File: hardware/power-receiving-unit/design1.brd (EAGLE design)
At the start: 55 x 40 mm, 99 parts, among them IC3 TPS54308DDCR, IC4 MCP6486T-E/OT, Q1 BSS138, Q2 SI3481DV, Y1 32MHz, Y2 32.768kHz

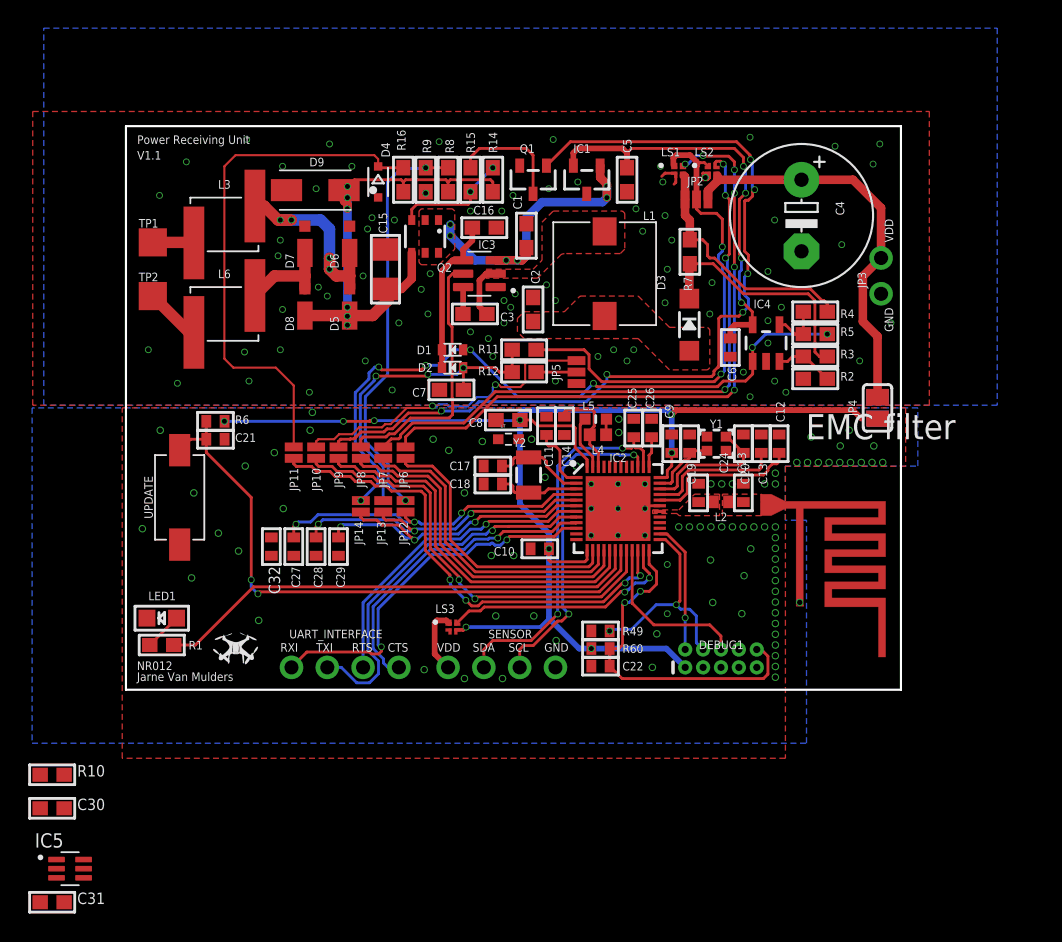
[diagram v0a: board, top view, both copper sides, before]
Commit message: Update hardware PTU
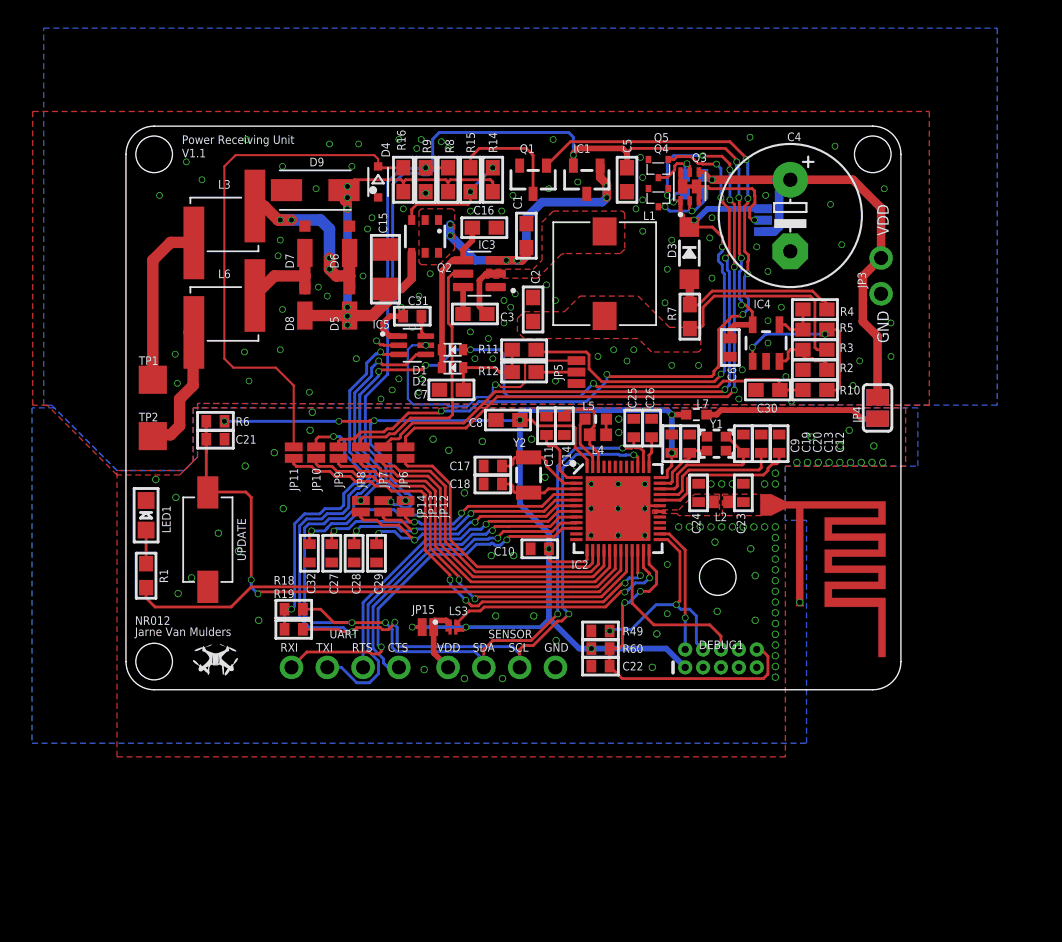
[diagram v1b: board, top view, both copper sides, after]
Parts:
- removed LS1, LS2: MIC94081YFT-TR, MIC94081YFT-TR:IC_MIC94081YFT-TR
- added JP15: JUMPER-SMT_2_NO_NO-SILK, SparkFun-Jumpers:SMT-JUMPER_2_NO_NO-SILK
- added Q3: PMDPB55XP, PMDPB55XP:SON65P200X200X65-8N
- added Q4, Q5: DMG1012T, microbuilder:SOT523-3
- added R13, R17: 100k, microbuilder:0402
- added R18, R19: 4k7, microbuilder:0402
- C23: value DNP -> 0.8p
- C31: device microbuilder:0603 -> microbuilder:0402
- moved R10 60.6 mm to (48.9, 21.3), turned to 180 degrees
- moved C30 58.8 mm to (45.6, 21.3)
- moved C31 48.8 mm to (20.3, 26.5)
- moved IC5 44.4 mm to (20.3, 24.4)
- moved L7 13.4 mm to (40.5, 19.5), turned to 180 degrees
- moved TP2 9.94 mm to (1.91, 18.0)
- moved TP1 9.75 mm to (1.91, 22.0)
- moved LED1 7.39 mm to (1.43, 12.4), turned to 0 degrees
- moved D3 5.08 mm to (40.0, 31.0)
- moved R1 5.05 mm to (1.43, 8.10), turned to 270 degrees
- moved JP2 4.94 mm to (45.2, 33.3), flipped to the bottom, turned to 270 degrees
- moved R7 4.60 mm to (40.0, 26.5)
- moved UPDATE 3.61 mm to (5.81, 10.7)
- moved C27 2.74 mm to (14.6, 9.68)
- moved C29 2.74 mm to (17.8, 9.68)
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- renumbered UART_INTERFACE to UART
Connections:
- removed net N$13: C2.1, D3.A, L1.2
- removed net PWM-CHG: IC5.5, JP10.2, JP5.3
- new net DIGI-POT: IC5.5, JP5.3
- new net I2C_PULLUP: JP10.2, R18.1, R19.1
- new net N$1: JP2.2, Q3.3, Q3.6, Q3.7, Q3.8
- new net N$17: Q3.2, Q4.3, R17.2
- new net N$18: Q3.5, Q5.3, R13.2
- new net OPAMP-OUT: IC4.1, R10.1, R5.2
- net AGND: now also Q4.2, Q5.2; no longer LS1.2, LS2.2
- net BUCK-OUT-1: now also C2.1, L1.2; no longer D3.C
- net BUCK-OUT-2: now also D3.A; no longer JP2.1, LS1.3
- net EN1: now also Q4.1; no longer LS1.4
- net EN2: now also Q5.1; no longer LS2.4
- net I2C_SCL: now also R19.2
- net I2C_SDA: now also R18.2
- net V-ICHG: no longer IC4.1, R10.1, R5.2
- net VCHG: now also Q3.4, R13.1; no longer LS2.3
- net VDD_BLE: now also JP15.1
- net VDD_SENS: now also JP15.2
- net VMEAS: now also D3.C, JP2.1, Q3.1, R17.1; no longer JP2.2, LS1.1, LS2.1
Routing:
- net I2C_SCL: track 22.9 -> 70.9 mm, vias 2 -> 5
- net I2C_SDA: track 26.6 -> 72.4 mm, vias 2 -> 5
- net 3.3V: track 29.8 -> 59.3 mm, vias 4 -> 6
- net PWM-CHG: track 22.5 -> 0.00 mm, vias 2 -> 0
- net I2C_PULLUP: track 0.00 -> 20.7 mm, vias 0 -> 2
- net DIGI-POT: track 0.00 -> 19.6 mm, vias 0 -> 2
- net V-VCHG: track 23.3 -> 6.79 mm, vias 3 -> 0
- net OPAMP-OUT: track 0.00 -> 12.8 mm, vias 0 -> 2
- net N$7: track 0.00 -> 12.5 mm
- net N$1: track 0.00 -> 10.5 mm, vias 0 -> 1
- net P19: track 34.7 -> 44.6 mm, vias 4 -> 6
- net N$14: track 2.93 -> 11.9 mm
- net N$12: track 3.98 -> 9.68 mm
- net N$17: track 0.00 -> 5.01 mm, vias 0 -> 2
- net VCHG: track 29.1 -> 34.1 mm, vias 0 -> 1
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- added copper zone on layer 1, net BUCK-OUT-1
- removed copper zone on layer 1, net N$13
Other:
- outline, holes or cut-outs redrawn
- board text removed: "EMC filter"

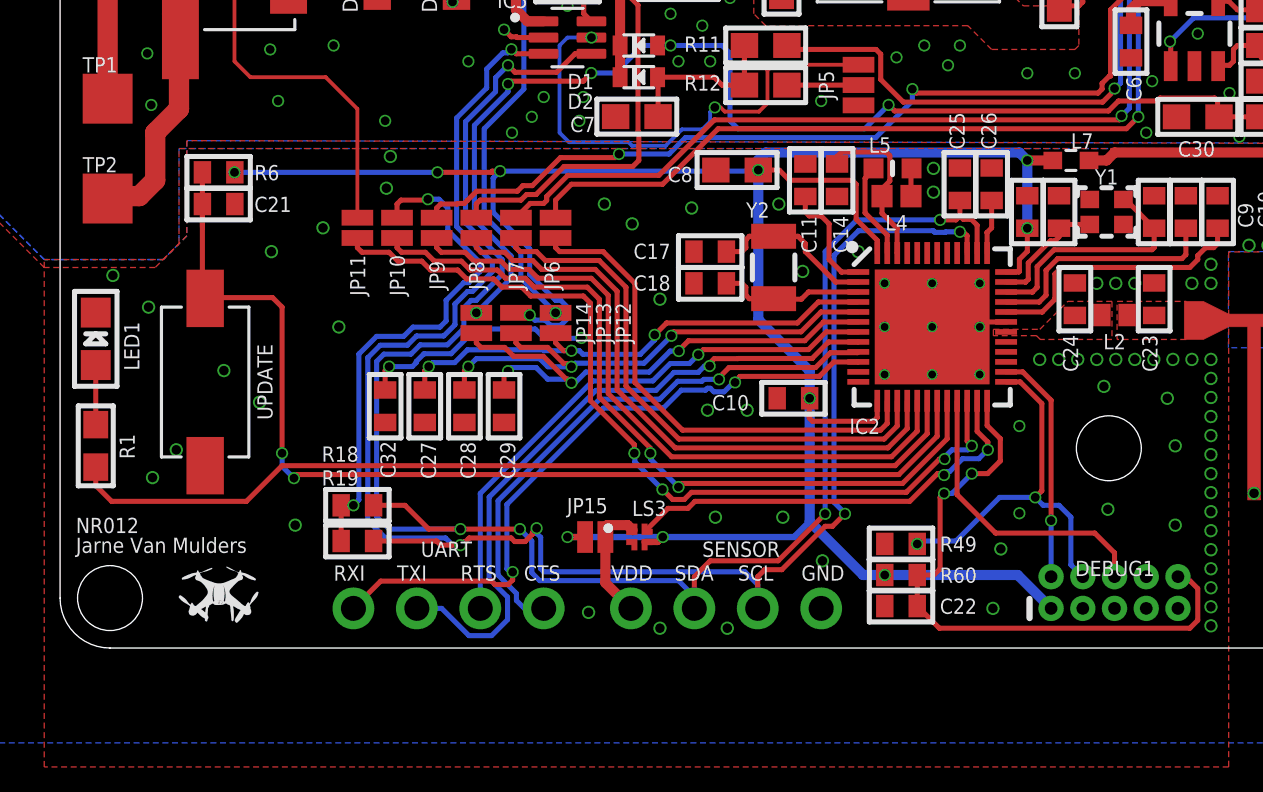
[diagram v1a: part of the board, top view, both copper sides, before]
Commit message: Update PTU firmware and hardware
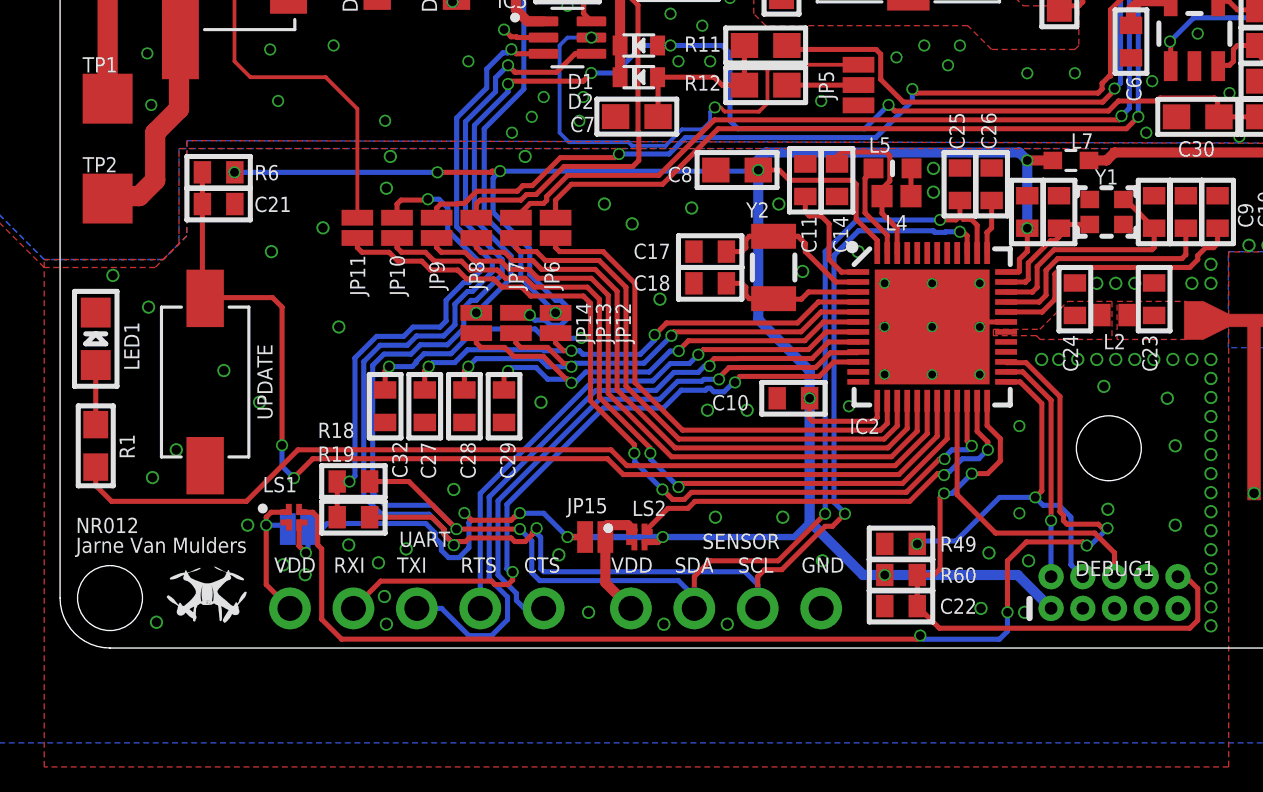
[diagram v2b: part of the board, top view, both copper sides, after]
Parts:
- added JP17: JUMPER-SMT_2_NO_NO-SILK, SparkFun-Jumpers:SMT-JUMPER_2_NO_NO-SILK
- added LS1: MIC94081YFT-TR, MIC94081YFT-TR:IC_MIC94081YFT-TR
- UART: device microbuilder:1X04_ROUND -> microbuilder:1X05_ROUND
- moved UART 1.27 mm to (14.3, 1.59)
- moved R18 0.97 mm to (11.7, 6.67)
- moved R19 0.97 mm to (11.7, 5.24)
- renumbered LS3 to LS2
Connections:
- removed net P22: IC2.27
- new net EN_MDM: IC2.27, LS1.4
- new net VDD_MDM: JP17.2, LS1.1, UART.1
- net GND: now also LS1.2
- net P05: now also UART.4; no longer UART.3
- net P06: now also UART.3; no longer UART.2
- net P07: now also UART.5; no longer UART.4
- net P08: now also UART.2; no longer UART.1
- net VDD_BLE: now also JP17.1, LS1.3
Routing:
- net EN_MDM: track 0.00 -> 50.2 mm, vias 0 -> 4
- net VDD_BLE: track 97.5 -> 113.7 mm, vias 11 -> 14
- net VDD_MDM: track 0.00 -> 5.97 mm, vias 0 -> 1
- net I2C_PULLUP: track 20.7 -> 19.8 mm
- net LED: track 36.7 -> 37.3 mm
- net GND: vias 91 -> 106
